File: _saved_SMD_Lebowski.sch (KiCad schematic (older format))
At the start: 43 parts, among them U1 PIC30F4011

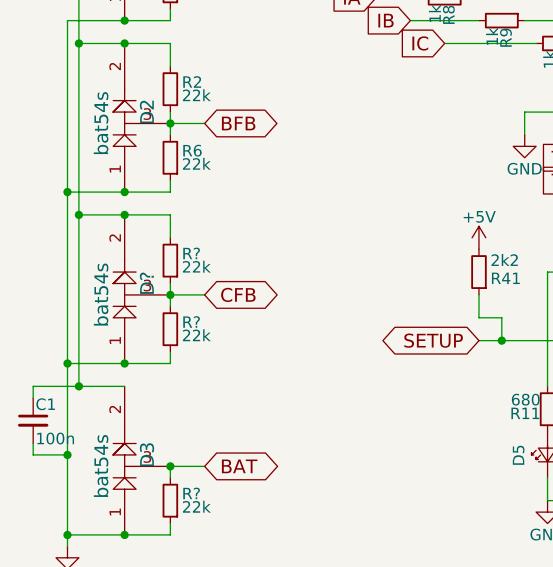
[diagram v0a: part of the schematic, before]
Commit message: work 06/20
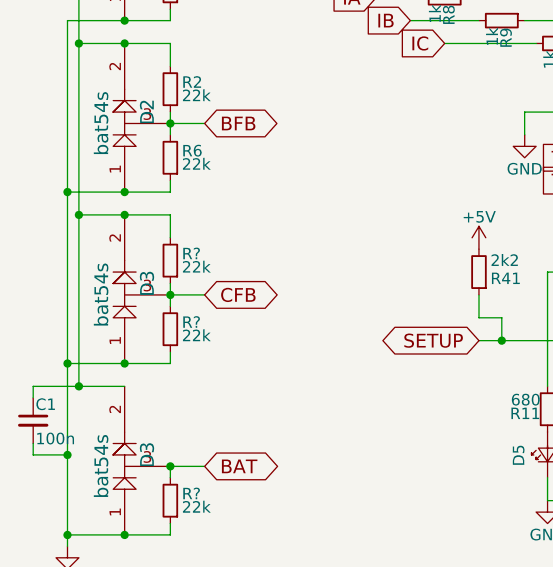
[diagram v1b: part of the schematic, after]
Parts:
- gave numbers to parts that had none: 1
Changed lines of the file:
@@
 $EndComp
 $Comp
-L bat54s D?
+L bat54s D3
 U 1 1 5B2B79EA
 P 1350 2750
-F 0 "D?" H 1400 2650 60  0000 C CNN
+F 0 "D3" H 1400 2650 60  0000 C CNN
 F 1 "bat54s" H 1350 2850 60  0000 C CNN
 F 2 "" H 1350 2750 60  0001 C CNN
